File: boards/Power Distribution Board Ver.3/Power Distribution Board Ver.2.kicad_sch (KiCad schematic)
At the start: 74 parts, among them J1 Screw_Terminal_01x02, J4 Screw_Terminal_01x06, U1 SIC431AED-T1-GE3, U2 SIC431AED-T1-GE3, U3 SIC431AED-T1-GE3

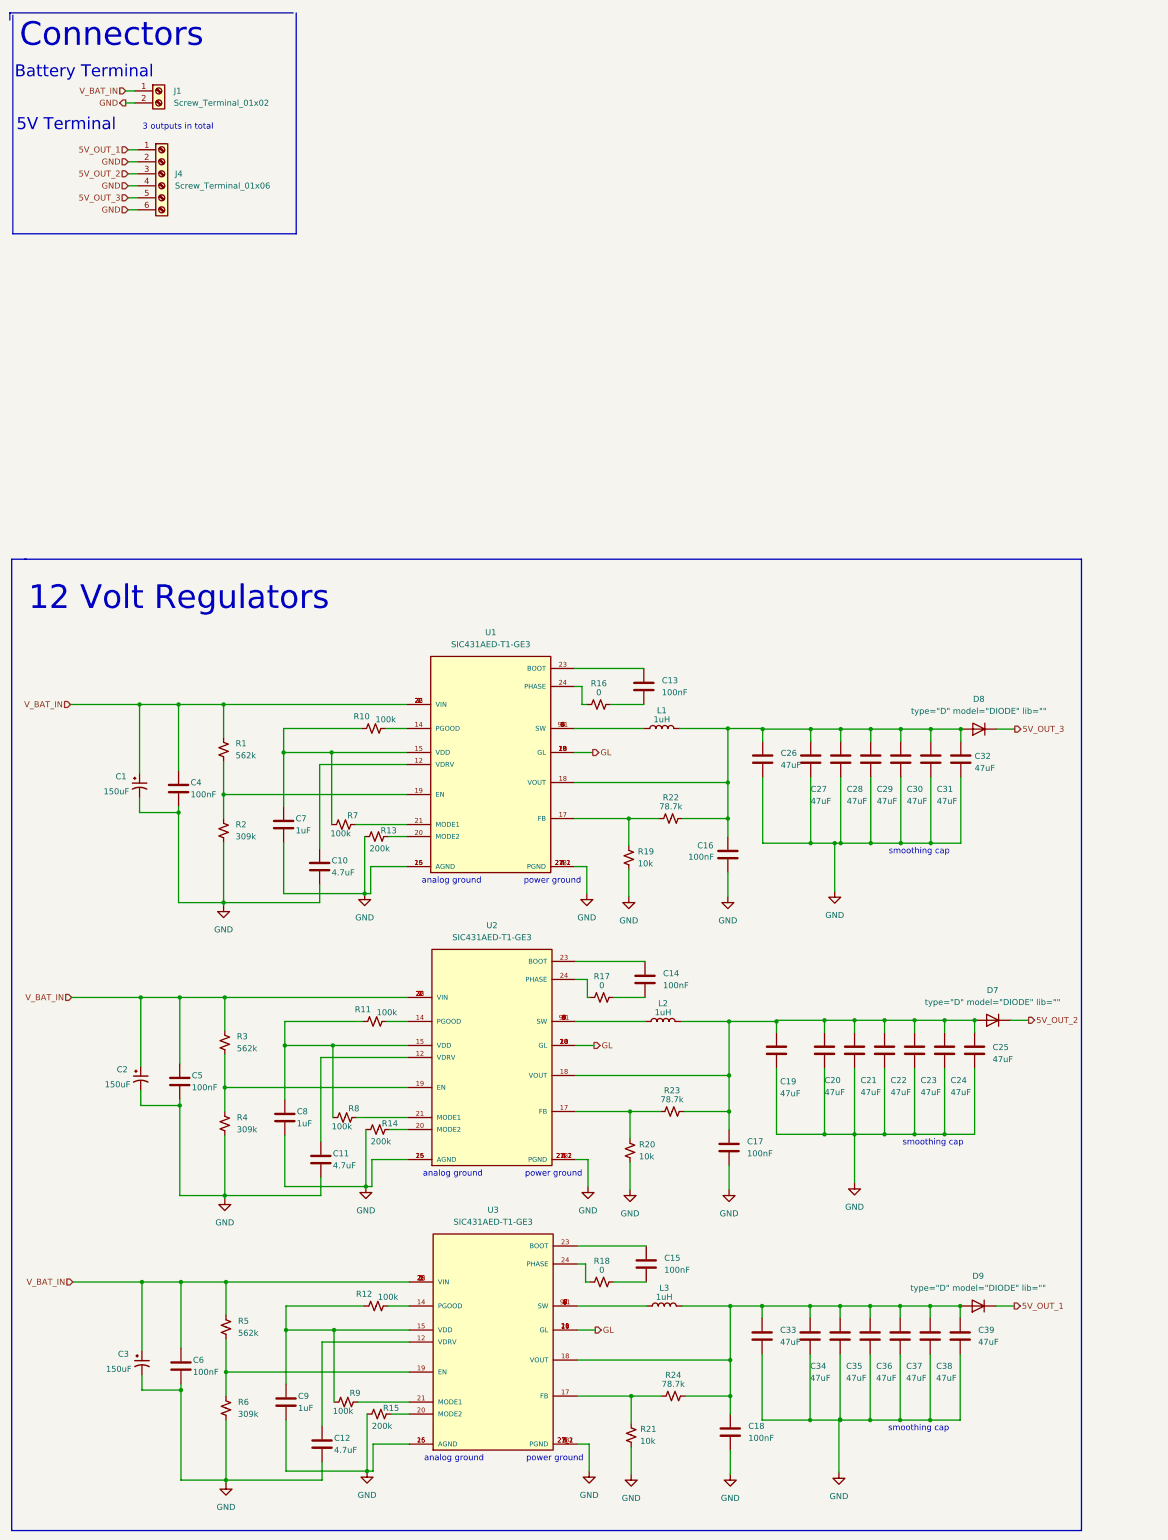
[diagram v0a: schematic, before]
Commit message: schematic changes
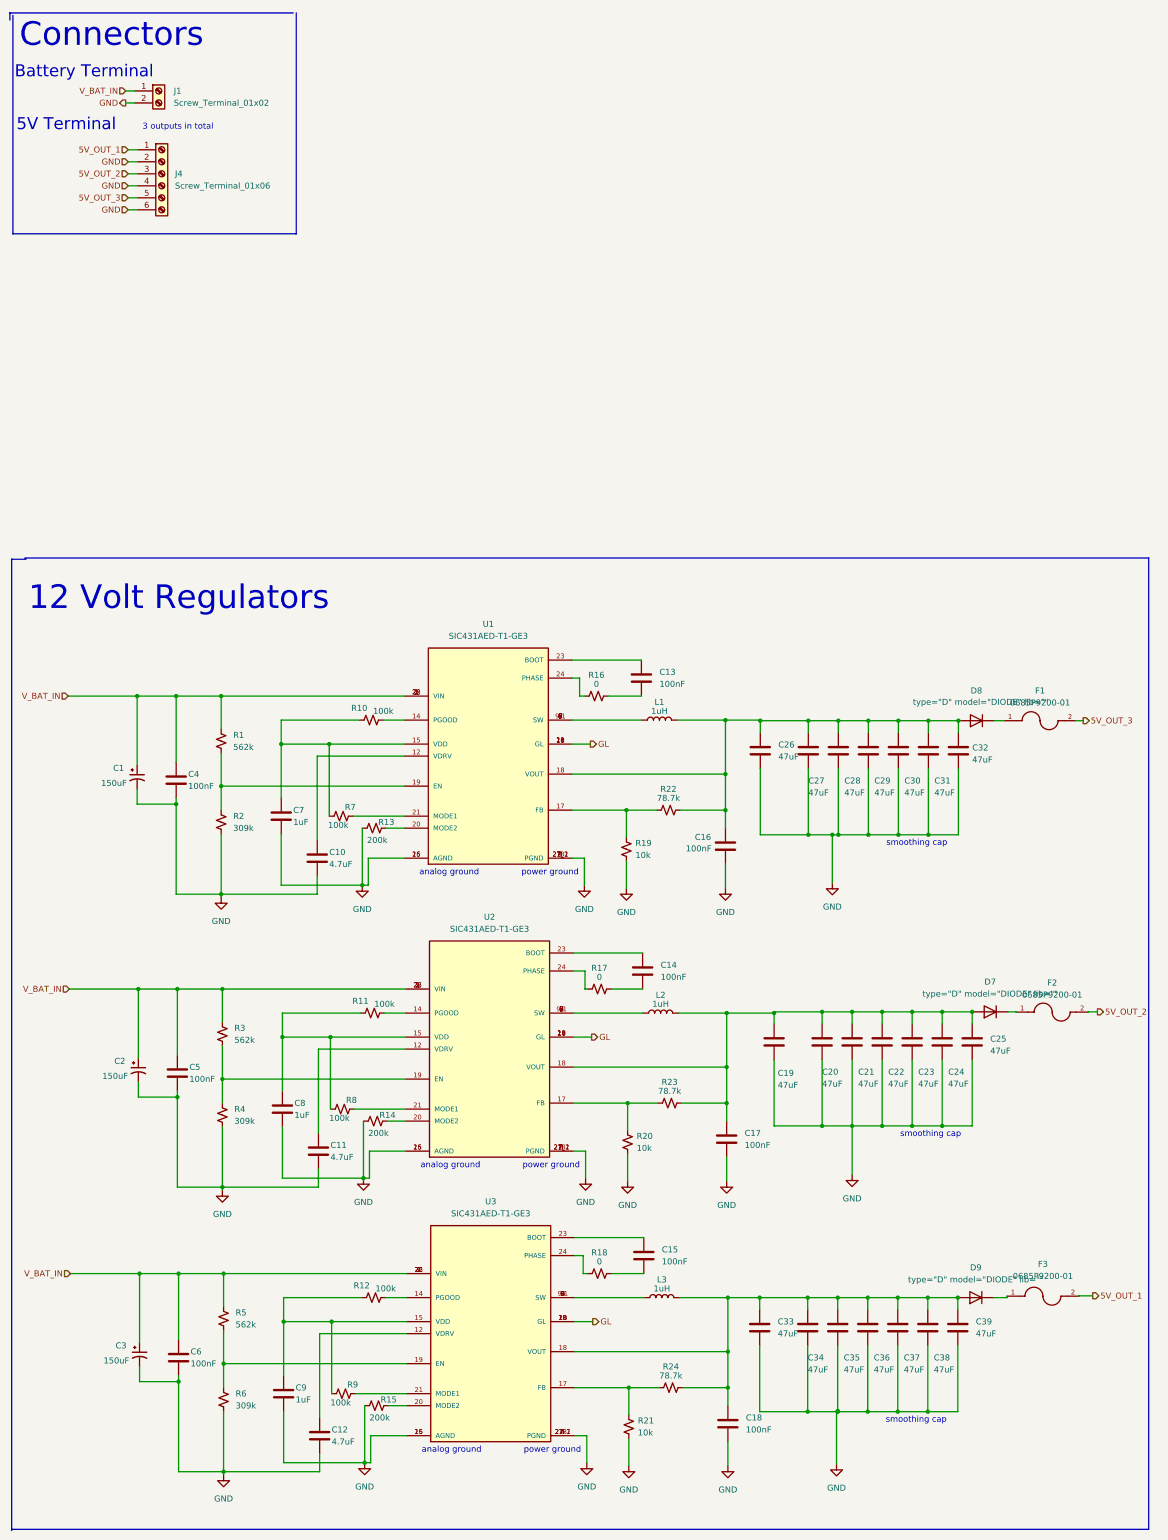
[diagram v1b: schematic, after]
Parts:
- added F1, F2, F3: 0685P9200-01, IRIS:FUSC3215X83N, symbol IRIS:0685P9200-01
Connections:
- net 5V_OUT_1: now also F3.2; no longer D9.2 (K)
- net 5V_OUT_2: now also F2.2; no longer D7.2 (K)
- net 5V_OUT_3: now also F1.2; no longer D8.2 (K)
- new net: D9.2 (K), F3.1
- new net: D8.2 (K), F1.1
- new net: D7.2 (K), F2.1
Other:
- moved on the sheet: C1, C10, C11, C12, C13, C14, C15, C16, C17, C18, C19, C2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

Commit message: PCBPCB Schematics Done
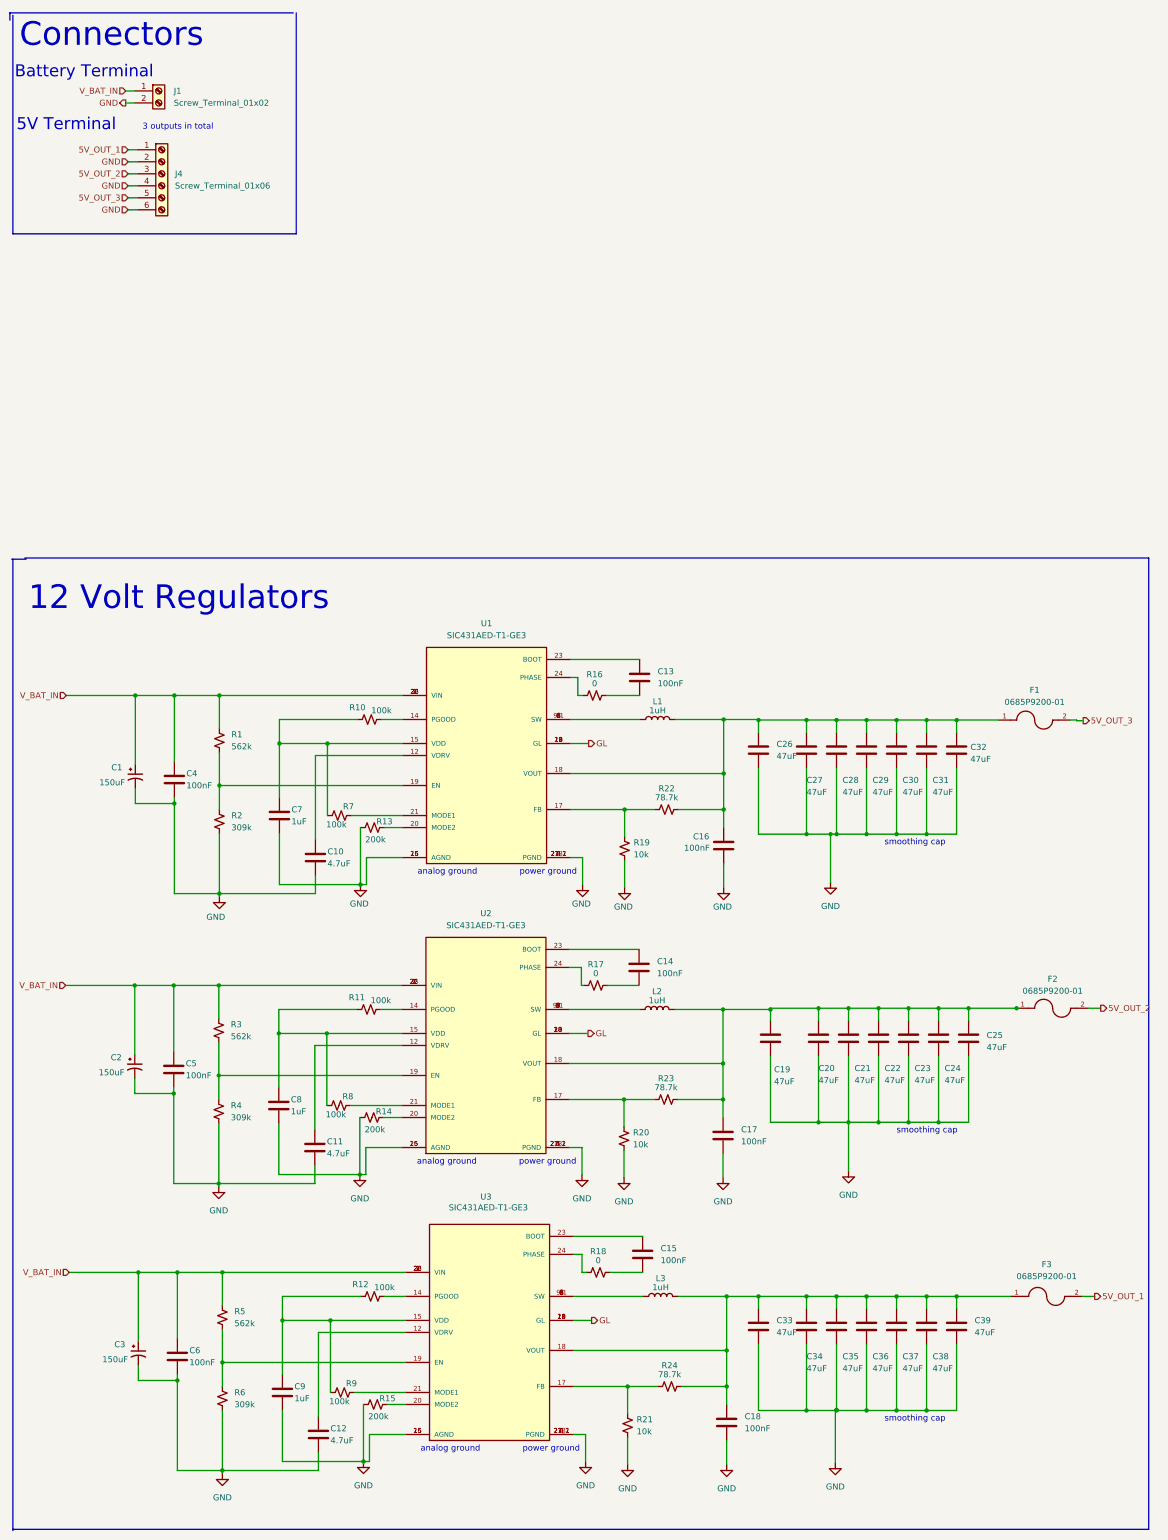
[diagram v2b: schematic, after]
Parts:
- removed D7, D8, D9: ${SIM.PARAMS}, Package_TO_SOT_SMD:TO-263-2, symbol Simulation_SPICE:DIODE
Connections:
- net at C18.1, C33.1, C34.1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: now also F3.1
- net at C16.1, C26.1, C27.1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: now also F1.1
- net at C17.1, C19.1, C20.1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: now also F2.1
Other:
- moved on the sheet: C11, C14, C17, C19, C2, C20, C21, C22, C23, C24, C25, C5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
